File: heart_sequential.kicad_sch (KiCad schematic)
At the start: 46 parts, among them SW1 SW_SPST, U1 NA555P, U2 4017

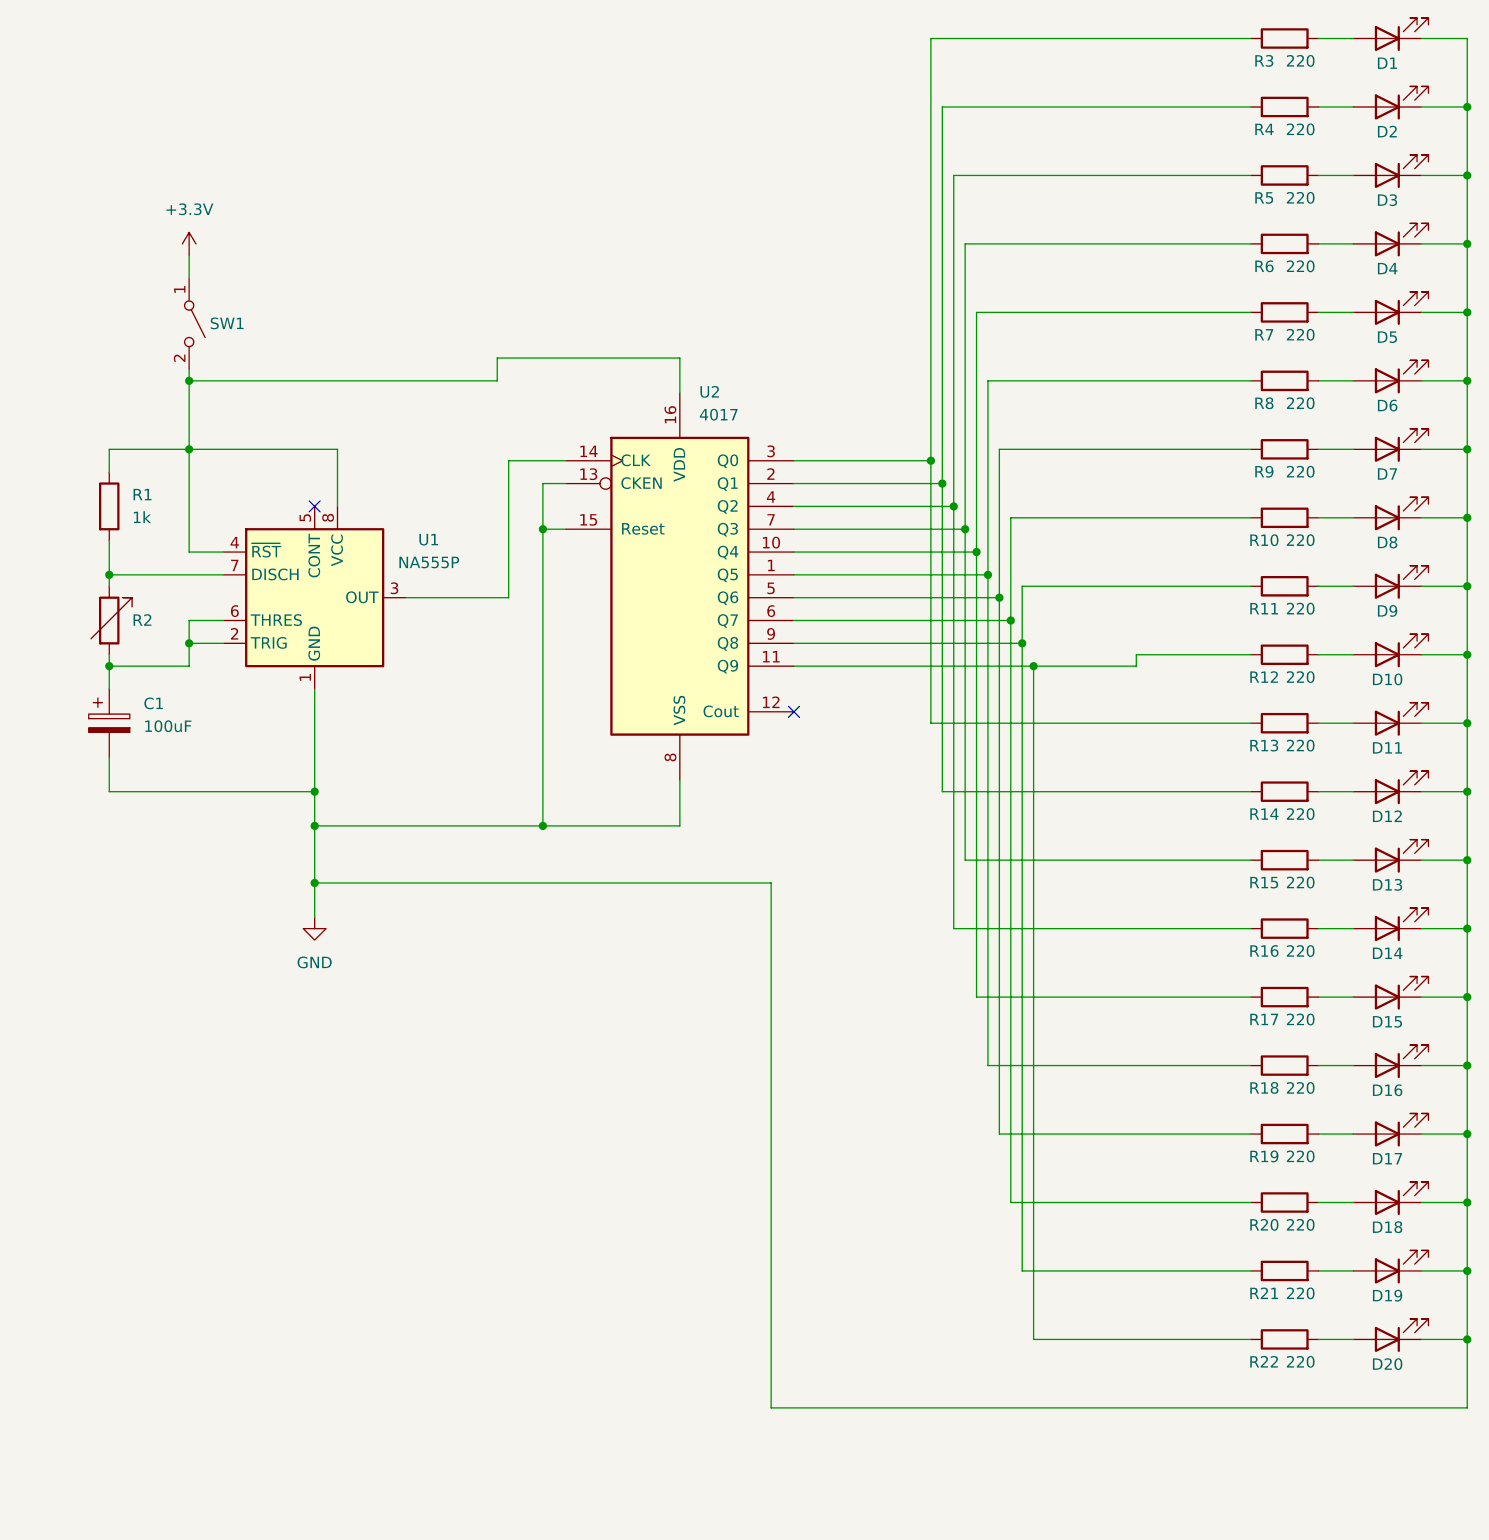
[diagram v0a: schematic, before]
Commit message: Update schematic
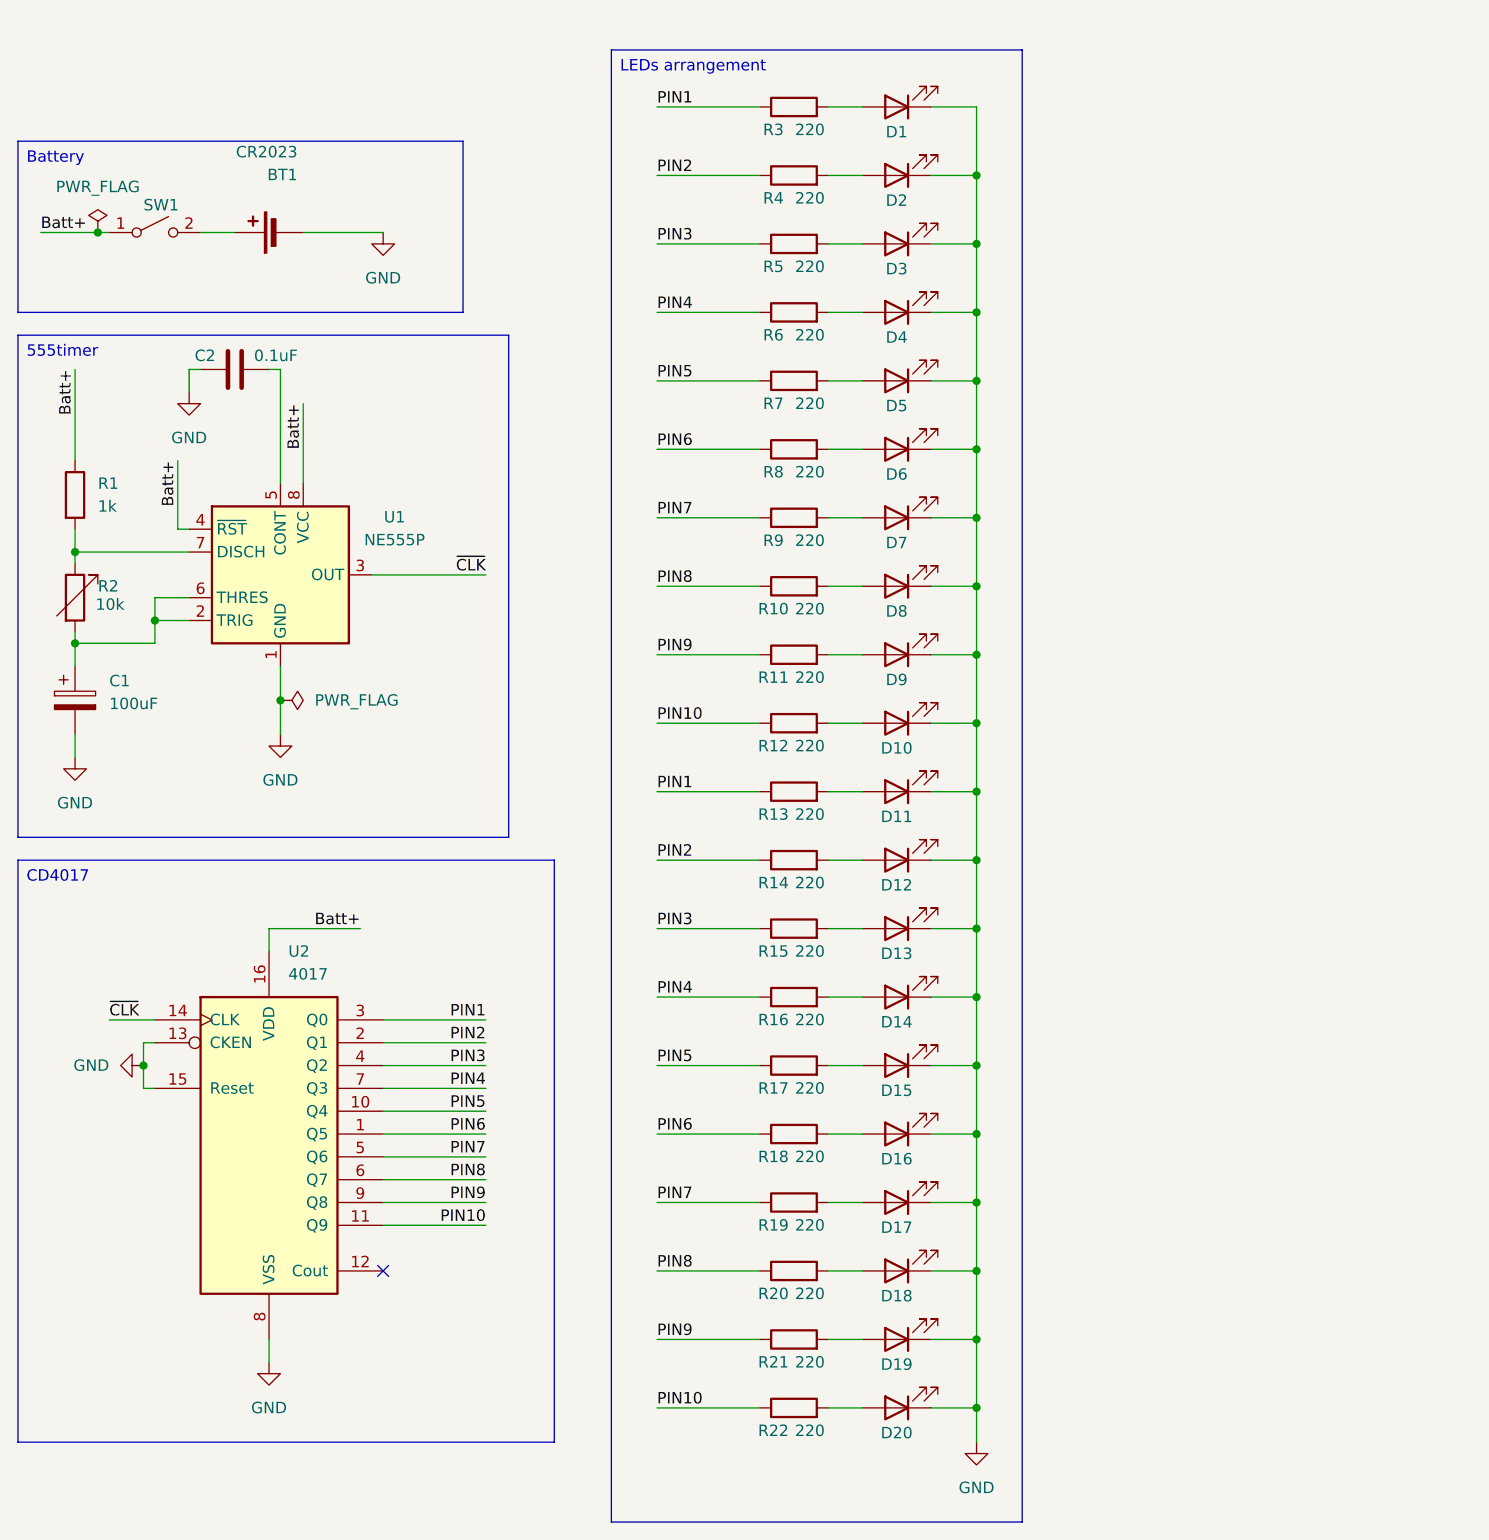
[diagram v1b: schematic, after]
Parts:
- removed U1: NA555P, Package_DIP:DIP-8_W7.62mm, symbol Timer:NA555P
- added BT1: CR2023, Battery:BatteryHolder_Keystone_2479_3xAAA, symbol Device:Battery_Cell
- added C2: 0.1uF, Capacitor_THT:C_Disc_D5.0mm_W2.5mm_P2.50mm, symbol Device:C
- added U1: NE555P, Package_DIP:DIP-8_W7.62mm, symbol Timer:NE555P
- R2: value R_Variable -> 10k
- SW1: footprint (none) -> Button_Switch_THT:SW_Slide_SPDT_Straight_CK_OS102011MS2Q
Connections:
- net +3.3V is gone; now on net Batt+: SW1.1 (A)
- net GND: now also BT1.2 (-), C2.1, U1.1 (GND)
- net PIN3: now reaches R5.1, U2.4 (Q2)
- net PIN3: now also R15.1; no longer R16.1
- net PIN8: now reaches R10.1, R20.1, U2.6 (Q7)
- net Batt+: now reaches R1.1, U2.16 (VDD)
- net Batt+: now also U1.4 (~{RST}), U1.8 (VCC); no longer SW1.2 (B)
- net at R1.2, R2.1: now also U1.7 (DISCH)
- net PIN9: now reaches R11.1, R21.1, U2.9 (Q8)
- net PIN1: now reaches R13.1, R3.1, U2.3 (Q0)
- net PIN6: now reaches R18.1, R8.1, U2.1 (Q5)
- net PIN5: now reaches R17.1, R7.1, U2.10 (Q4)
- net PIN10: now reaches R12.1, R22.1, U2.11 (Q9)
- net ~{CLK}: now reaches U2.14 (CLK)
- net ~{CLK}: now also U1.3 (OUT)
- net PIN2: now reaches R14.1, R4.1, U2.2 (Q1)
- net PIN7: now reaches R19.1, R9.1, U2.5 (Q6)
- net PIN4: now reaches R6.1, U2.7 (Q3)
- net PIN4: now also R16.1; no longer R15.1
- net at C1.1, R2.2: now also U1.2 (TRIG), U1.6 (THRES)
- new net: BT1.1 (+), SW1.2 (B)
- new net: C2.2, U1.5 (CONT)
- no-connect marks 2 -> 1
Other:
- moved on the sheet: C1, D1, D2, R1, R10, R11, R12, R13, R14, R15, R16, R17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
